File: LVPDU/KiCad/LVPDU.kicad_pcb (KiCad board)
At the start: 2 copper layers, 12 parts, among them J1 Conn_01x14, K1 T9VV1K15-12S

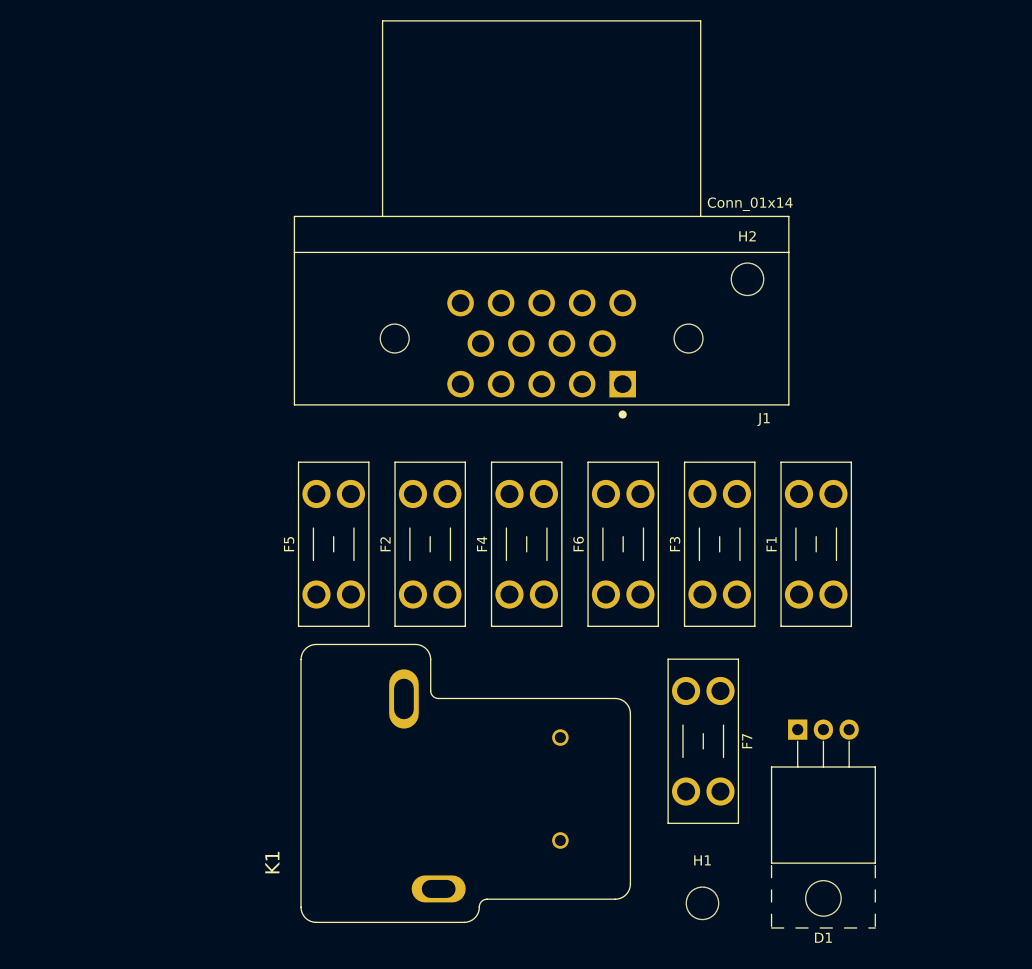
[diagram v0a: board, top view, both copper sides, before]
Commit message: first board rev
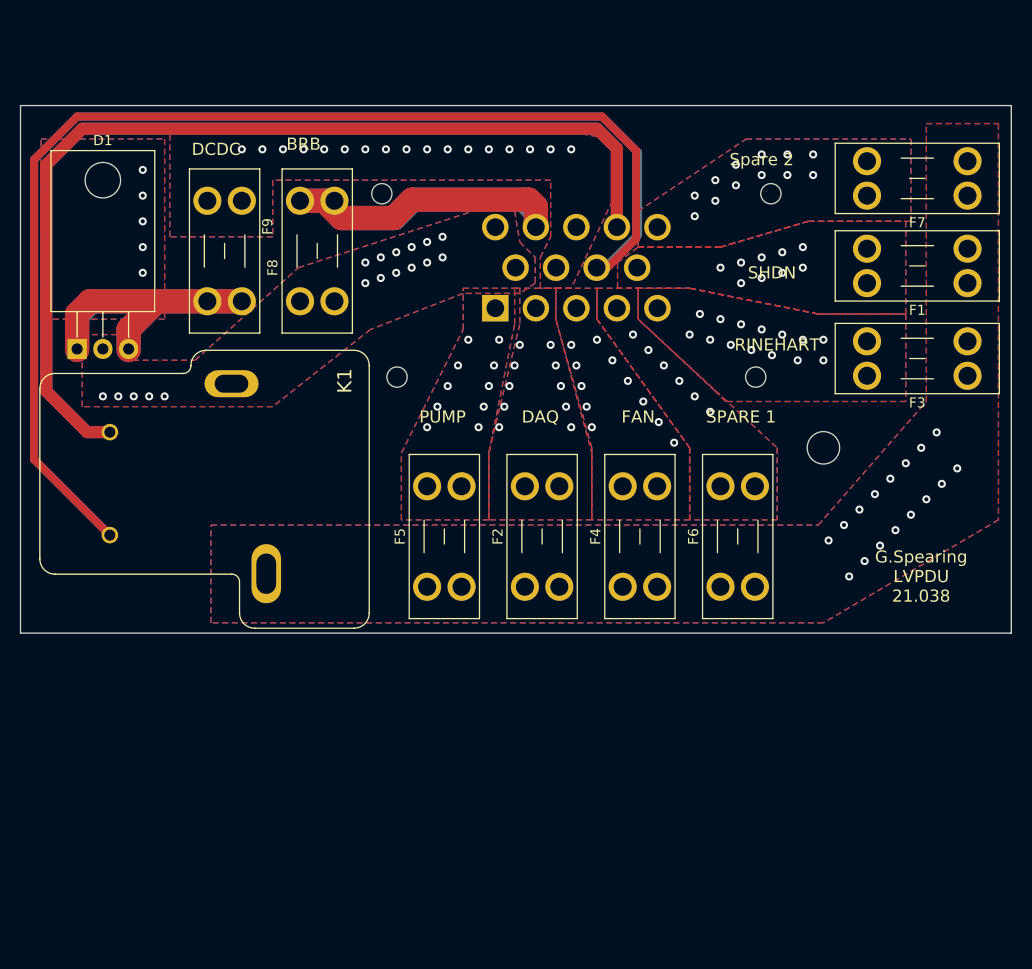
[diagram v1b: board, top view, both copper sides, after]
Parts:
- removed H2: MountingHole, MountingHole:MountingHole_3.2mm_M3
- added F8: 3568 Mini Blade, AERO_CUSTOM:Fuseholder_Blade_Mini_Keystone_3568, F.Cu at (173.2, 46.2)
- added F9: 3568 Mini Blade, AERO_CUSTOM:Fuseholder_Blade_Mini_Keystone_3568, F.Cu at (164.1, 46.2)
- D1: footprint Package_TO_SOT_THT:TO-220-3_Horizontal_TabUp -> Package_TO_SOT_THT:TO-220-3_Horizontal_TabDown
- J1: footprint AERO_CUSTOM:TE_1-776266-1_14pin_Horizontal -> AERO_CUSTOM:TE_1-776262-1_14pin_Vertical; moved to B.Cu
- moved D1 80.4 mm to (147.8, 60.9)
- moved F7 54.6 mm to (235.7, 45.7), turned to 180 degrees
- moved H1 46.5 mm to (221.5, 70.6)
- moved K1 37.2 mm to (163.1, 73.7), turned to 270 degrees
- moved F1 34.9 mm to (235.7, 54.4), turned to 180 degrees
- moved F3 33.9 mm to (235.7, 63.5), turned to 180 degrees
- moved F6 11.3 mm to (211.3, 84.3)
- moved F4 11.2 mm to (201.7, 84.3)
- moved F2 11.1 mm to (192.0, 84.3)
- moved F5 10.9 mm to (182.4, 84.3)
- moved J1 8.24 mm to (197.1, 52.8), turned to 0 degrees
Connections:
- D1 pad 1: /DCDC_IN -> /DCDC_Fused
- D1 pad 3: /DCDC_IN -> /DCDC_Fused
- F6 pad 2: /12V_OUT -> /12V_OUT_1
- F7 pad 1: /TO_BRB -> +12V
- F7 pad 2: /BATT_IN -> /12V_OUT_2
- J1 pad 1: /SHUTDOWN_OUT -> /PUMP
- J1 pad 11: /BATT_IN -> /TO_BRB
- J1 pad 13: /DCDC_IN -> /FROM_BRB
- J1 pad 14: GND -> /12V_OUT_2
- J1 pad 3: /RINEHART -> /RADIATOR
- J1 pad 4: /RADIATOR -> /12V_OUT_1
- J1 pad 5: /PUMP -> /RINEHART
- J1 pad 6: /12V_OUT -> /BATT_IN
- J1 pad 7: /12V_OUT -> /DCDC_IN
- J1 pad 8: /TO_BRB -> GND
- J1 pad 9: /FROM_BRB -> /SHUTDOWN_OUT
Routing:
- net GND: track 0.00 -> 233.1 mm
- net /FROM_BRB: track 0.00 -> 193.3 mm
- net /TO_BRB: track 0.00 -> 55.8 mm
- net /DCDC_Fused: track 0.00 -> 52.5 mm
- net /SHUTDOWN_OUT: vias 0 -> 9
- net /RINEHART: vias 0 -> 14
- net /RADIATOR: vias 0 -> 11
- net /PUMP: vias 0 -> 10
- net /DCDC_IN: vias 0 -> 17
- net /DAQ: vias 0 -> 10
- net /BATT_IN: vias 0 -> 17
- net /12V_OUT_2: vias 0 -> 12
- net /12V_OUT_1: vias 0 -> 6
- net +12V: vias 0 -> 16
- net (no net): vias 0 -> 5
- added copper zone on B.Cu, net +12V
- added copper zone on F.Cu, net +12V
- added copper zone on B.Cu, net /12V_OUT_1
- added copper zone on F.Cu, net /12V_OUT_1
- added copper zone on B.Cu, net /12V_OUT_2
- added copper zone on F.Cu, net /12V_OUT_2
- added copper zone on B.Cu, net /BATT_IN
- added copper zone on F.Cu, net /BATT_IN
- added copper zone on B.Cu, net /DAQ
- added copper zone on F.Cu, net /DAQ
- added copper zone on B.Cu, net /DCDC_IN
- added copper zone on F.Cu, net /DCDC_IN
- added copper zone on B.Cu, net /PUMP
- added copper zone on F.Cu, net /PUMP
- added copper zone on B.Cu, net /RADIATOR
- added copper zone on F.Cu, net /RADIATOR
- added copper zone on B.Cu, net /RINEHART
- added copper zone on F.Cu, net /RINEHART
- added copper zone on B.Cu, net /SHUTDOWN_OUT
- added copper zone on F.Cu, net /SHUTDOWN_OUT
- added copper zone on B.Cu, net GND
- added copper zone on F.Cu, net GND
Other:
- board outline added: 97.8 x 52.1 mm
- board text added: "BRB"
- board text added: "DAQ"
- board text added: "DCDC"
- board text added: "FAN"
- board text added: "G.Spearing LVPDU 21.038"
- board text added: "PUMP"
- board text added: "RINEHART"
- board text added: "SHDN"
- board text added: "SPARE 1"
- board text added: "Spare 2"
